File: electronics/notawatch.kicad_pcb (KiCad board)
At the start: 2 copper layers, 44 x 40 mm, 26 parts, among them SW1 SW_Push, SW2 SW_Push, SW3 SW_Push, SW4 SW_Push, U1 ATtiny84A-SSU, U2 DS1307Z+, U3 HT16K33-24, U4 KWM-20882AVB, U5 SPX3819M5-L-5-0, Y1 32768Hz

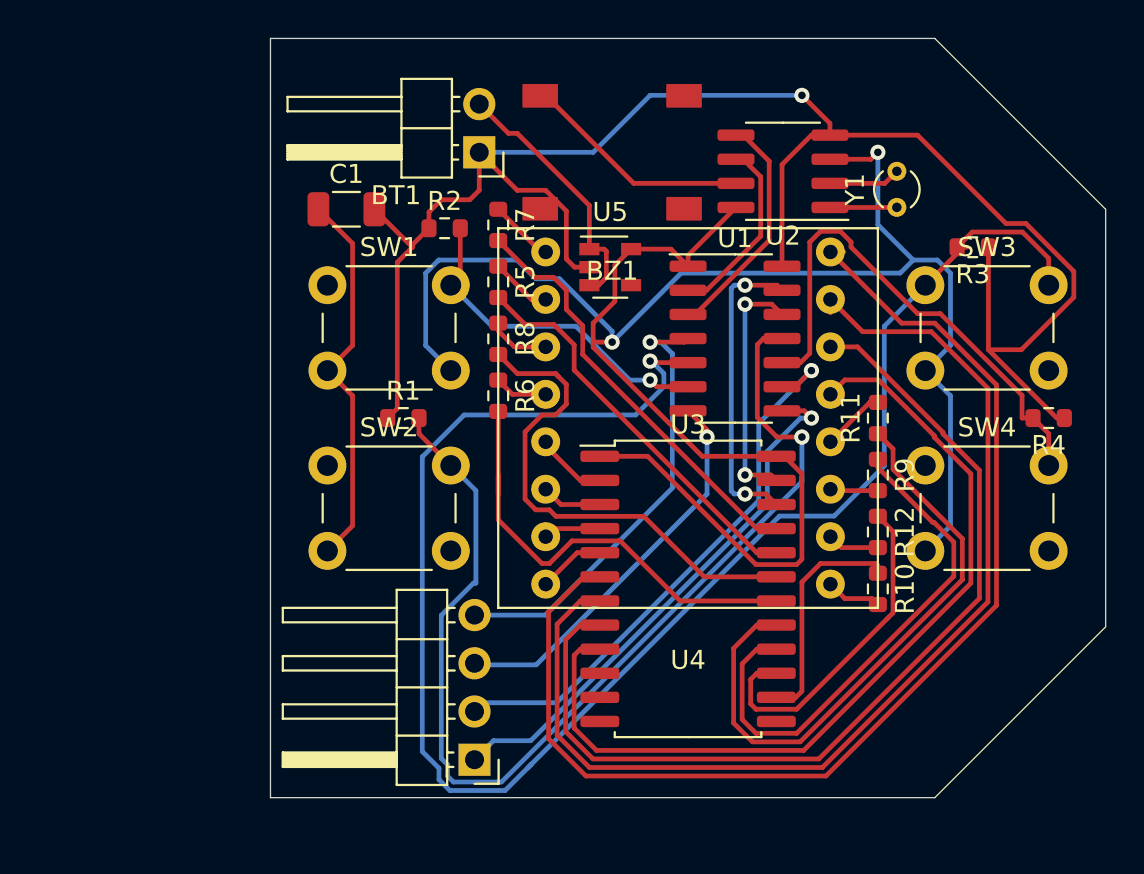
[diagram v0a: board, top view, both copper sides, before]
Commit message: Trust me, I'm usually more dilligent about documenting git changes
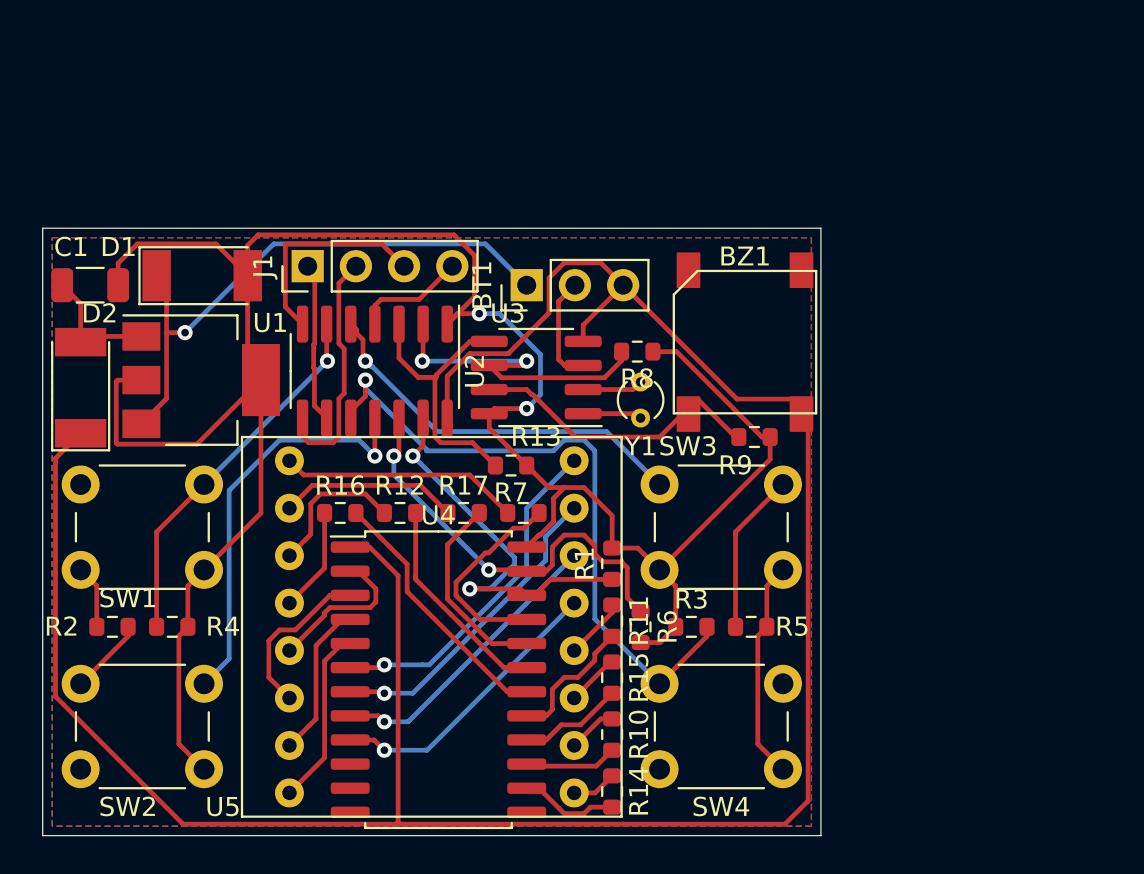
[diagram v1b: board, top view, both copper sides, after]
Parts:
- removed REF**: PinHeader_1x04_P2.54mm_Horizontal, Connector_PinHeader_2.54mm:PinHeader_1x04_P2.54mm_Horizontal
- added D1: SM4007, Diode_SMD:D_MELF, F.Cu at (126.4, 95.5)
- added D2: SM4007, Diode_SMD:D_MELF, F.Cu at (120.0, 101.4)
- added J1: Conn_01x04, Connector_PinHeader_2.54mm:PinHeader_1x04_P2.54mm_Vertical, F.Cu at (132.0, 95.0)
- added R13: 470, Resistor_SMD:R_0603_1608Metric, F.Cu at (143.3, 108.0)
- added R14: 470, Resistor_SMD:R_0603_1608Metric, F.Cu at (148.0, 122.7)
- added R15: 470, Resistor_SMD:R_0603_1608Metric, F.Cu at (148.0, 116.7)
- added R16: 470, Resistor_SMD:R_0603_1608Metric, F.Cu at (133.7, 108.0)
- added R17: 470, Resistor_SMD:R_0603_1608Metric, F.Cu at (140.2, 108.0)
- BT1: value 6V -> Double_Battery_Cell; footprint Connector_PinHeader_2.54mm:PinHeader_1x02_P2.54mm_Horizontal -> Connector_PinHeader_2.54mm:PinHeader_1x03_P2.54mm_Vertical
- C1: value 2.2uF -> 22uF
- R5, R6, R7, R8, R9: value 470 -> 10k
- U1: value ATtiny84A-SSU -> AMS1117-5.0; footprint Package_SO:SOIC-14_3.9x8.7mm_P1.27mm -> Package_TO_SOT_SMD:SOT-223-3_TabPin2
- U2: value DS1307Z+ -> ATtiny84A-SSU; footprint Package_SO:SOIC-8_3.9x4.9mm_P1.27mm -> Package_SO:SOIC-14_3.9x8.7mm_P1.27mm
- U3: value HT16K33-24 -> DS1307ZN+; footprint Package_SO:SOIC-24W_7.5x15.4mm_P1.27mm -> Package_SO:SOIC-8_3.9x4.9mm_P1.27mm
- U4: value KWM-20882AVB -> HT16K33-24; footprint LED_matrix:KVM-20882AVB -> Package_SO:SOIC-24W_7.5x15.4mm_P1.27mm
- U5: value SPX3819M5-L-5-0 -> KWM-20882AVB; footprint Package_TO_SOT_SMD:SOT-23-5 -> LED_matrix:KVM-20882AVB
- moved R4 47.5 mm to (124.8, 114.0)
- moved U1 28.2 mm to (126.3, 101.0)
- moved R2 27.3 mm to (121.7, 114.0)
- moved R12 25.2 mm to (136.8, 108.0), turned to 0 degrees
- moved R3 24.9 mm to (152.2, 114.0), turned to 0 degrees
- moved U2 23.9 mm to (135.5, 100.5), turned to -90 degrees
- moved R5 22.5 mm to (155.3, 114.0), turned to 180 degrees
- moved U5 21.2 mm to (138.5, 114.0)
- moved U4 19.1 mm to (138.8, 116.8)
- moved SW4 18.1 mm to (150.5, 117.0)
- moved R11 17.6 mm to (148.0, 113.7), turned to -90 degrees
- moved SW3 17.5 mm to (150.5, 106.5)
- moved Y1 17.5 mm to (149.5, 103.0)
- moved SW2 17.4 mm to (120.0, 117.0)
- moved SW1 16.7 mm to (120.0, 106.5)
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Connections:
- BT1 pad 1: GND -> +BATT
- BT1 pad 2: Net-(BT1-Pad1) -> +3V3
- C1 pad 2: GND -> Net-(C1-Pad2)
- R1 pad 1: GND -> Net-(R1-Pad1)
- R1 pad 2: Net-(R1-Pad2) -> +5V
- R2 pad 1: GND -> +5V
- R3 pad 1: GND -> +5V
- R4 pad 1: GND -> +5V
- R5 pad 1: Net-(R5-Pad1) -> +5V
- R6 pad 2: Net-(R6-Pad2) -> +5V
- R7 pad 1: Net-(R7-Pad1) -> +5V
- R8 pad 1: Net-(R8-Pad1) -> +5V
- R9 pad 1: Net-(R9-Pad1) -> +5V
- R9 pad 2: Net-(R9-Pad2) -> Net-(BZ1-Pad1)
- SW1 pad 1: Net-(R2-Pad2) -> Net-(R4-Pad2)
- SW2 pad 1: Net-(R1-Pad2) -> Net-(R2-Pad2)
- SW3 pad 1: Net-(R3-Pad2) -> Net-(R5-Pad2)
- SW4 pad 1: Net-(R4-Pad2) -> Net-(R3-Pad2)
- U1 pad 1: +5V -> Net-(C1-Pad2)
- U1 pad 2: Net-(U1-Pad2) -> +5V
- U1 pad 3: Net-(U1-Pad3) -> +BATT
- U2 pad 1: Net-(U2-Pad1) -> +5V
- U2 pad 2: Net-(U2-Pad2) -> Net-(R8-Pad2)
- U2 pad 3: +5V -> Net-(R7-Pad2)
- U2 pad 4: GND -> Net-(J1-Pad4)
- U2 pad 5: Net-(U1-Pad3) -> Net-(R5-Pad2)
- U2 pad 6: Net-(U1-Pad2) -> Net-(R4-Pad2)
- U2 pad 7: Net-(BZ1-Pad1) -> Net-(J1-Pad3)
- U2 pad 8: +5V -> Net-(J1-Pad2)
- U3 pad 1: +5V -> Net-(U3-Pad1)
- U3 pad 3: Net-(U3-Pad3) -> +3V3
- U3 pad 4: Net-(U3-Pad4) -> GND
- U3 pad 5: Net-(U3-Pad5) -> Net-(R7-Pad2)
- U3 pad 6: Net-(U3-Pad6) -> Net-(R8-Pad2)
- U3 pad 7: Net-(U3-Pad7) -> Net-(BZ1-Pad1)
- U3 pad 8: Net-(U3-Pad8) -> +5V
- U4 pad 1: Net-(R7-Pad1) -> GND
- U4 pad 10: Net-(R12-Pad2) -> Net-(U4-Pad10)
- U4 pad 11: Net-(R9-Pad2) -> Net-(U4-Pad11)
- U4 pad 12: Net-(R11-Pad2) -> Net-(U4-Pad12)
- U4 pad 13: Net-(U3-Pad9) -> Net-(U4-Pad13)
- U4 pad 14: Net-(U3-Pad8) -> Net-(R14-Pad2)
- U4 pad 15: Net-(U3-Pad7) -> Net-(R10-Pad2)
- U4 pad 16: Net-(U3-Pad6) -> Net-(R15-Pad2)
- U4 pad 2: Net-(R5-Pad1) -> Net-(U4-Pad2)
- U4 pad 3: Net-(R8-Pad1) -> Net-(U4-Pad3)
- U4 pad 4: Net-(R6-Pad1) -> Net-(U4-Pad4)
- U4 pad 5: Net-(U3-Pad2) -> Net-(U4-Pad5)
- U4 pad 6: Net-(U3-Pad3) -> Net-(U4-Pad6)
- U4 pad 7: Net-(U3-Pad4) -> Net-(U4-Pad7)
- U4 pad 8: Net-(U3-Pad5) -> Net-(U4-Pad8)
- U4 pad 9: Net-(R10-Pad2) -> Net-(U4-Pad9)
- U5 pad 1: Net-(BT1-Pad1) -> Net-(R13-Pad1)
- U5 pad 2: GND -> Net-(R17-Pad1)
- U5 pad 3: Net-(BT1-Pad1) -> Net-(R12-Pad1)
- U5 pad 5: +5V -> Net-(U4-Pad2)
- Y1 pad 1: Net-(U2-Pad1) -> Net-(U3-Pad1)
- Y1 pad 2: Net-(U2-Pad2) -> Net-(U3-Pad2)
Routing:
- net Net-(U3-Pad6): track 62.3 -> 0.00 mm
- net Net-(U3-Pad7): track 57.8 -> 0.00 mm
- net Net-(R1-Pad2): track 56.8 -> 0.00 mm, vias 1 -> 0
- net Net-(R3-Pad2): track 87.0 -> 34.4 mm
- net Net-(U3-Pad8): track 50.2 -> 0.00 mm
- net Net-(U3-Pad9): track 46.0 -> 0.00 mm
- net GND: track 93.6 -> 125.9 mm, vias 1 -> 0
- net +BATT: track 0.00 -> 30.4 mm, vias 0 -> 1
- net Net-(U1-Pad9): track 29.5 -> 0.00 mm, vias 1 -> 0
- net Net-(R11-Pad1): track 32.2 -> 3.23 mm
- net Net-(U1-Pad8): track 28.5 -> 0.00 mm, vias 1 -> 0
- net Net-(R9-Pad1): track 27.8 -> 0.00 mm
- net Net-(R6-Pad2): track 24.1 -> 0.00 mm
- net Net-(U1-Pad4): track 23.8 -> 0.00 mm, vias 1 -> 0
- net Net-(R1-Pad1): track 0.00 -> 21.0 mm, vias 0 -> 2
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- added copper zone on B.Cu, net (none)
- added copper zone on F.Cu, net (none)
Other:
- board size 44 x 40 mm -> 41 x 32 mm
- net class Default removed
